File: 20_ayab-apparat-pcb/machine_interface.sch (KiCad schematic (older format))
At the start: 12 parts, among them K1 CONN_3, K2 CONN_3, P1 CONN_4, P2 CONN_10, P3 CONN_10, P4 CONN_8, P5 CONN_5, P6 CONN_5, U2 PCF8574, U3 PCF8574, U4 ULN2803, U5 ULN2803

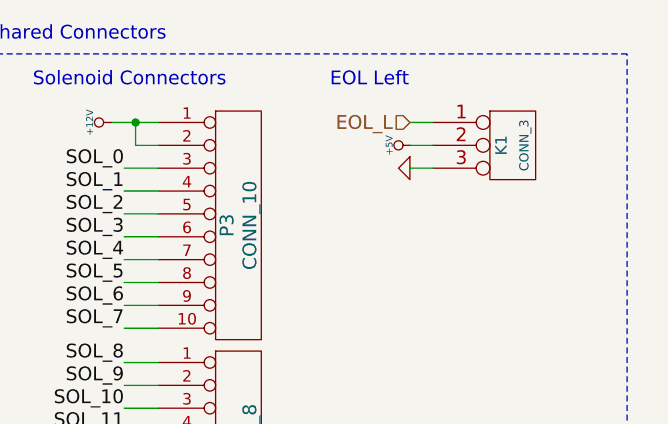
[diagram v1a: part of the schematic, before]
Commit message: ayab-apparat v2 ready for review
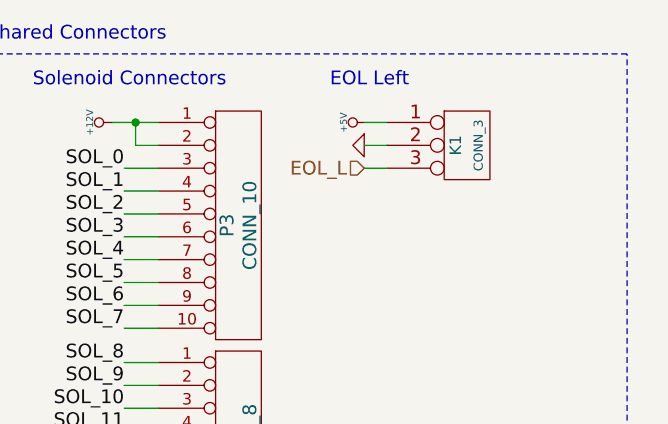
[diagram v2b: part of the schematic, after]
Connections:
- net +5V: now also K1.1 (P1); no longer K1.2 (PM)
- net EOL_L: now also K1.3 (P3); no longer K1.1 (P1)
- net GND: now also K1.2 (PM); no longer K1.3 (P3)
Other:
- moved on the sheet: K1
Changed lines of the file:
@@
 L CONN_3 K1
 U 1 1 52E14DD9
-P 8100 1550
-F 0 "K1" V 8050 1550 50  0000 C CNN
-F 1 "CONN_3" V 8150 1550 40  0000 C CNN
-F 2 "" H 8100 1550 60  0000 C CNN
-F 3 "" H 8100 1550 60  0000 C CNN
-	1    8100 1550
+P 7900 1550
+F 0 "K1" V 7850 1550 50  0000 C CNN
+F 1 "CONN_3" V 7950 1550 40  0000 C CNN
+F 2 "" H 7900 1550 60  0000 C CNN
+F 3 "" H 7900 1550 60  0000 C CNN
+	1    7900 1550
 	1    0    0    -1
 $EndComp
@@
 	1    0    0    -1
 $EndComp
-Text HLabel 7650 1450 0    60   Input ~ 0
+Text HLabel 7450 1650 0    60   Input ~ 0
 EOL_L
 $Comp
 L +5V #PWR08
 U 1 1 52E1540D
-P 7650 1550
-F 0 "#PWR08" H 7650 1640 20  0001 C CNN
-F 1 "+5V" H 7650 1640 30  0000 C CNN
-F 2 "" H 7650 1550 60  0000 C CNN
-F 3 "" H 7650 1550 60  0000 C CNN
-	1    7650 1550
+P 7450 1450
+F 0 "#PWR08" H 7450 1540 20  0001 C CNN
+F 1 "+5V" H 7450 1540 30  0000 C CNN
+F 2 "" H 7450 1450 60  0000 C CNN
+F 3 "" H 7450 1450 60  0000 C CNN
+	1    7450 1450
 	0    -1   -1   0
 $EndComp
@@
 L GND #PWR09
 U 1 1 52E15421
-P 7650 1650
-F 0 "#PWR09" H 7650 1650 30  0001 C CNN
-F 1 "GND" H 7650 1580 30  0001 C CNN
-F 2 "" H 7650 1650 60  0000 C CNN
-F 3 "" H 7650 1650 60  0000 C CNN
-	1    7650 1650
+P 7450 1550
+F 0 "#PWR09" H 7450 1550 30  0001 C CNN
+F 1 "GND" H 7450 1480 30  0001 C CNN
+F 2 "" H 7450 1550 60  0000 C CNN
+F 3 "" H 7450 1550 60  0000 C CNN
+	1    7450 1550
 	0    1    1    0
 $EndComp
@@
 V2
 Wire Wire Line
-	7650 1550 7750 1550
+	7450 1450 7550 1450
 Wire Wire Line
 	6300 4200 6500 4200
@@
 	6400 4300 6500 4300
 Wire Wire Line
-	7750 1650 7650 1650
-Wire Wire Line
-	7650 1450 7750 1450
+	7550 1550 7450 1550
+Wire Wire Line
+	7450 1650 7550 1650
 Wire Wire Line
 	6400 4000 6500 4000
